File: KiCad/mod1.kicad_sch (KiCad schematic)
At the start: 150 parts, among them J13 SFF-8654-8i, J14 RJE361882415, J17 Bus_PCI_Express_x4, J18 HDMI_A, M1 Fan_4pin, M2 Fan_4pin, Q4 2N7002, Q5 2N7002, Q6 2N7002, Q7 2N7002, U1 ZD25Q64BSIGT, U45 RTL8125BG-CG, U46 H5VU25U, U47 H5VU25U, U48 H5VU25U, U49 H5VU25U, U50 H5VU25U, U51 H5VU25U, U52 H5VU25U, U53 H5VU25U, Y7 25MHz

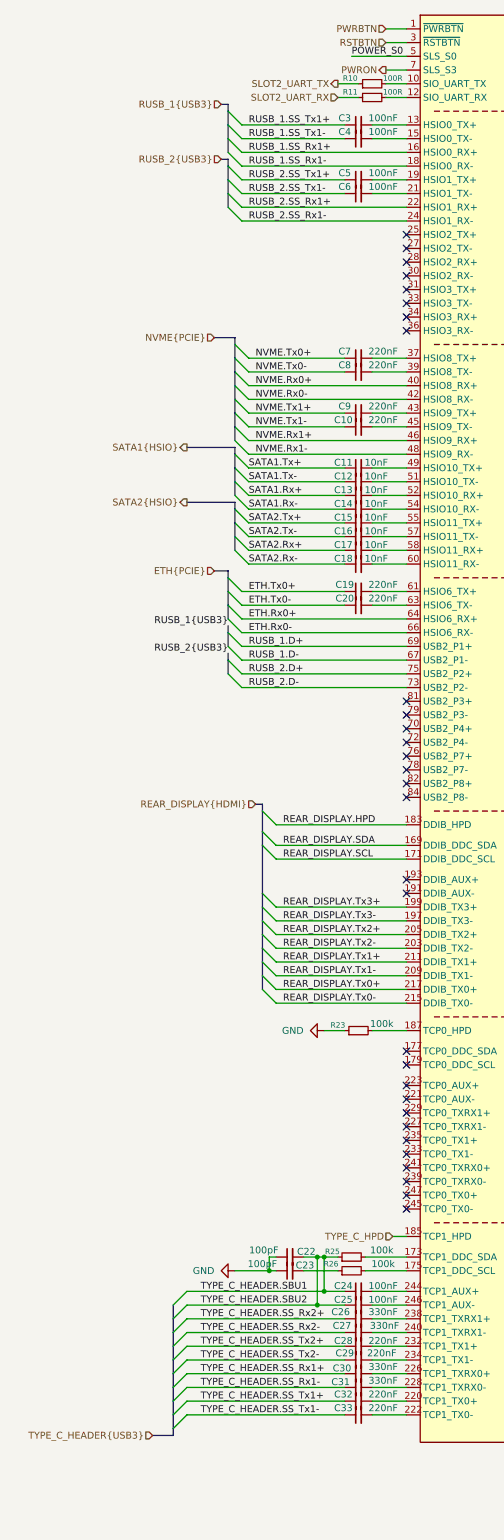
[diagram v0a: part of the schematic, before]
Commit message: Start connecting module
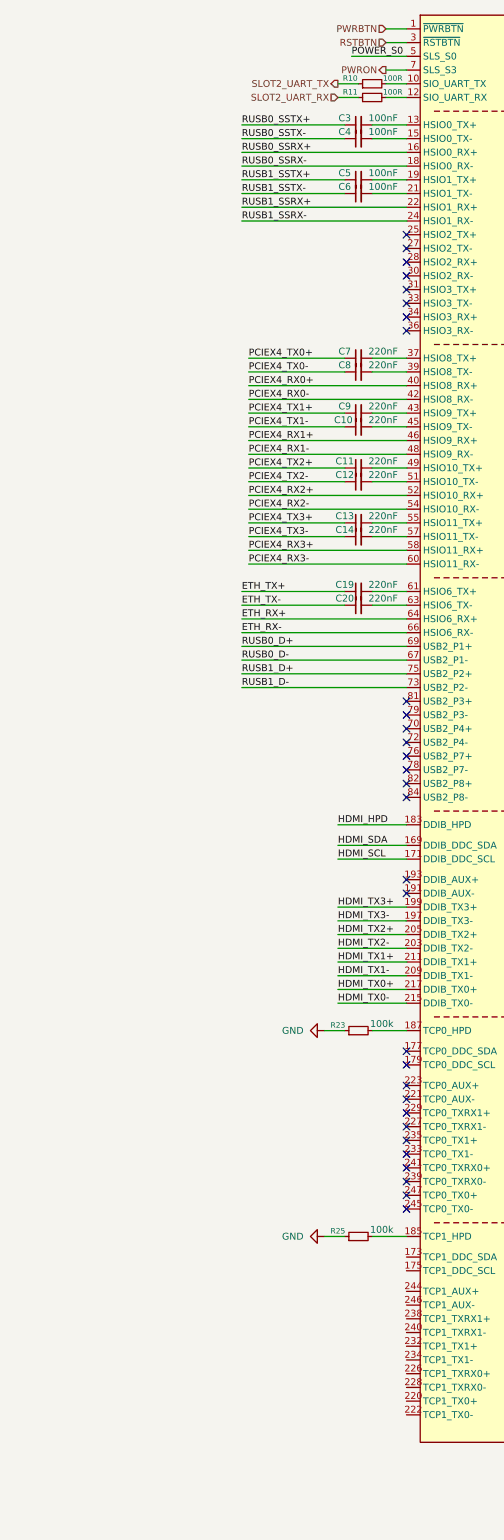
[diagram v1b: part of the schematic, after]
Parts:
- removed C15, C16, C17, C18: 10nF, Capacitor_SMD:C_0402_1005Metric, symbol Device:C_Small
- removed C22, C23: 100pF, Capacitor_SMD:C_0402_1005Metric, symbol Device:C_Small
- removed C24, C25: 100nF, Capacitor_SMD:C_0402_1005Metric, symbol Device:C_Small
- removed C26, C27, C30, C31: 330nF, Capacitor_SMD:C_0402_1005Metric, symbol Device:C_Small
- removed C28, C29, C32, C33: 220nF, Capacitor_SMD:C_0402_1005Metric, symbol Device:C_Small
- removed R26: 100k, Resistor_SMD:R_0402_1005Metric, symbol Device:R_Small
- C11, C12, C13, C14: value 10nF -> 220nF
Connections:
- net ETH.Rx0+ is gone; now on net ETH_RX+: A1.64 (HSIO6_RX+)
- net ETH.Rx0- is gone; now on net ETH_RX-: A1.66 (HSIO6_RX-)
- net ETH.Tx0+ is gone; now on net ETH_TX+: C19.1
- net ETH.Tx0- is gone; now on net ETH_TX-: C20.1
- net NVME.Rx0+ is gone; now on net PCIEX4_RX0+: A1.40 (HSIO8_RX+)
- net NVME.Rx0- is gone; now on net PCIEX4_RX0-: A1.42 (HSIO8_RX-)
- net NVME.Rx1+ is gone; now on net PCIEX4_RX1+: A1.46 (HSIO9_RX+)
- net NVME.Rx1- is gone; now on net PCIEX4_RX1-: A1.48 (HSIO9_RX-)
- net NVME.Tx0+ is gone; now on net PCIEX4_TX0+: C7.1
- net NVME.Tx0- is gone; now on net PCIEX4_TX0-: C8.1
- net NVME.Tx1+ is gone; now on net PCIEX4_TX1+: C9.1
- net NVME.Tx1- is gone; now on net PCIEX4_TX1-: C10.1
- net REAR_DISPLAY.HPD is gone; now on net HDMI_HPD: A1.183 (DDIB_HPD)
- net REAR_DISPLAY.SCL is gone; now on net HDMI_SCL: A1.171 (DDIB_DDC_SCL)
- net REAR_DISPLAY.SDA is gone; now on net HDMI_SDA: A1.169 (DDIB_DDC_SDA)
- net REAR_DISPLAY.Tx0+ is gone; now on net HDMI_TX0+: A1.217 (DDIB_TX0+)
- net REAR_DISPLAY.Tx0- is gone; now on net HDMI_TX0-: A1.215 (DDIB_TX0-)
- net REAR_DISPLAY.Tx1+ is gone; now on net HDMI_TX1+: A1.211 (DDIB_TX1+)
- net REAR_DISPLAY.Tx1- is gone; now on net HDMI_TX1-: A1.209 (DDIB_TX1-)
- net REAR_DISPLAY.Tx2+ is gone; now on net HDMI_TX2+: A1.205 (DDIB_TX2+)
- net REAR_DISPLAY.Tx2- is gone; now on net HDMI_TX2-: A1.203 (DDIB_TX2-)
- net REAR_DISPLAY.Tx3+ is gone; now on net HDMI_TX3+: A1.199 (DDIB_TX3+)
- net REAR_DISPLAY.Tx3- is gone; now on net HDMI_TX3-: A1.197 (DDIB_TX3-)
- net RUSB_1.D+ is gone; now on net RUSB0_D+: A1.69 (USB2_P1+)
- net RUSB_1.D- is gone; now on net RUSB0_D-: A1.67 (USB2_P1-)
- net RUSB_1.SS_Rx1+ is gone; now on net RUSB0_SSRX+: A1.16 (HSIO0_RX+)
- net RUSB_1.SS_Rx1- is gone; now on net RUSB0_SSRX-: A1.18 (HSIO0_RX-)
- net RUSB_1.SS_Tx1+ is gone; now on net RUSB0_SSTX+: C3.1
- net RUSB_1.SS_Tx1- is gone; now on net RUSB0_SSTX-: C4.1
- net RUSB_2.D+ is gone; now on net RUSB1_D+: A1.75 (USB2_P2+)
- net RUSB_2.D- is gone; now on net RUSB1_D-: A1.73 (USB2_P2-)
- net RUSB_2.SS_Rx1+ is gone; now on net RUSB1_SSRX+: A1.22 (HSIO1_RX+)
- net RUSB_2.SS_Rx1- is gone; now on net RUSB1_SSRX-: A1.24 (HSIO1_RX-)
- net RUSB_2.SS_Tx1+ is gone; now on net RUSB1_SSTX+: C5.1
- net RUSB_2.SS_Tx1- is gone; now on net RUSB1_SSTX-: C6.1
- net SATA1.Rx+ is gone; now on net PCIEX4_TX3+: C13.1
- net SATA1.Rx- is gone; now on net PCIEX4_TX3-: C14.1
- net SATA1.Tx+ is gone; now on net PCIEX4_TX2+: C11.1
- net SATA1.Tx- is gone; now on net PCIEX4_TX2-: C12.1
- net TYPE_C_HEADER.SBU1 is gone; now on net GND: R25.1
- net PCIEX4_RX2+: now also A1.52 (HSIO10_RX+)
- net PCIEX4_RX2-: now also A1.54 (HSIO10_RX-)
- net PCIEX4_RX3+: now also A1.58 (HSIO11_RX+)
- net PCIEX4_RX3-: now also A1.60 (HSIO11_RX-)
- net at C13.2: now also A1.55 (HSIO11_TX+); no longer A1.52 (HSIO10_RX+)
- net at A1.57 (HSIO11_TX-): now also C14.2
- net at A1.173 (TCP1_DDC_SDA): no longer R25.2
- net TYPE_C_HPD: no longer names the net of A1.185 (TCP1_HPD)
- net TYPE_C_HPD: now also R25.2
